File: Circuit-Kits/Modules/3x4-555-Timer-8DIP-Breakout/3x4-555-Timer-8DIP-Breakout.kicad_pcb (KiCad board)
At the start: 2 copper layers, 23.6 x 31.6 mm, 1 part, among them U1 555TIMER

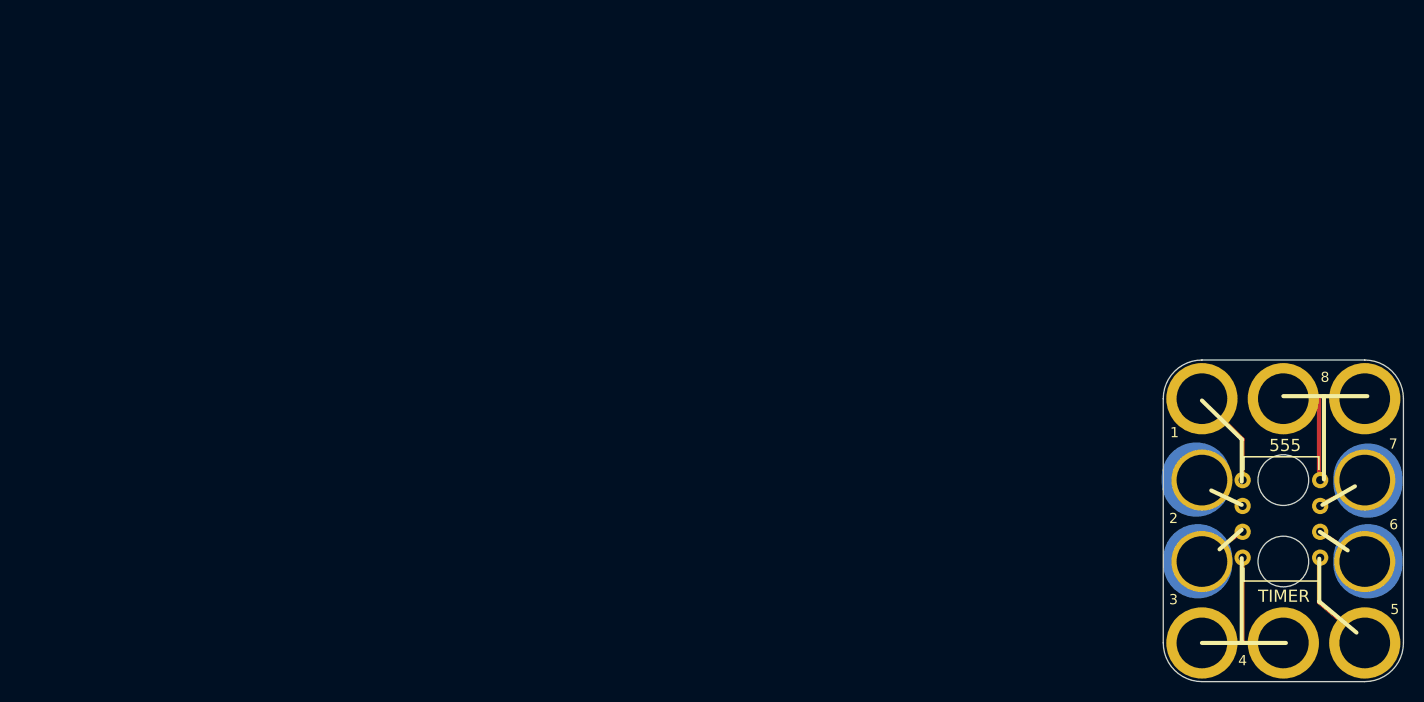
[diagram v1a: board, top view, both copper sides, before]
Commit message: Public release
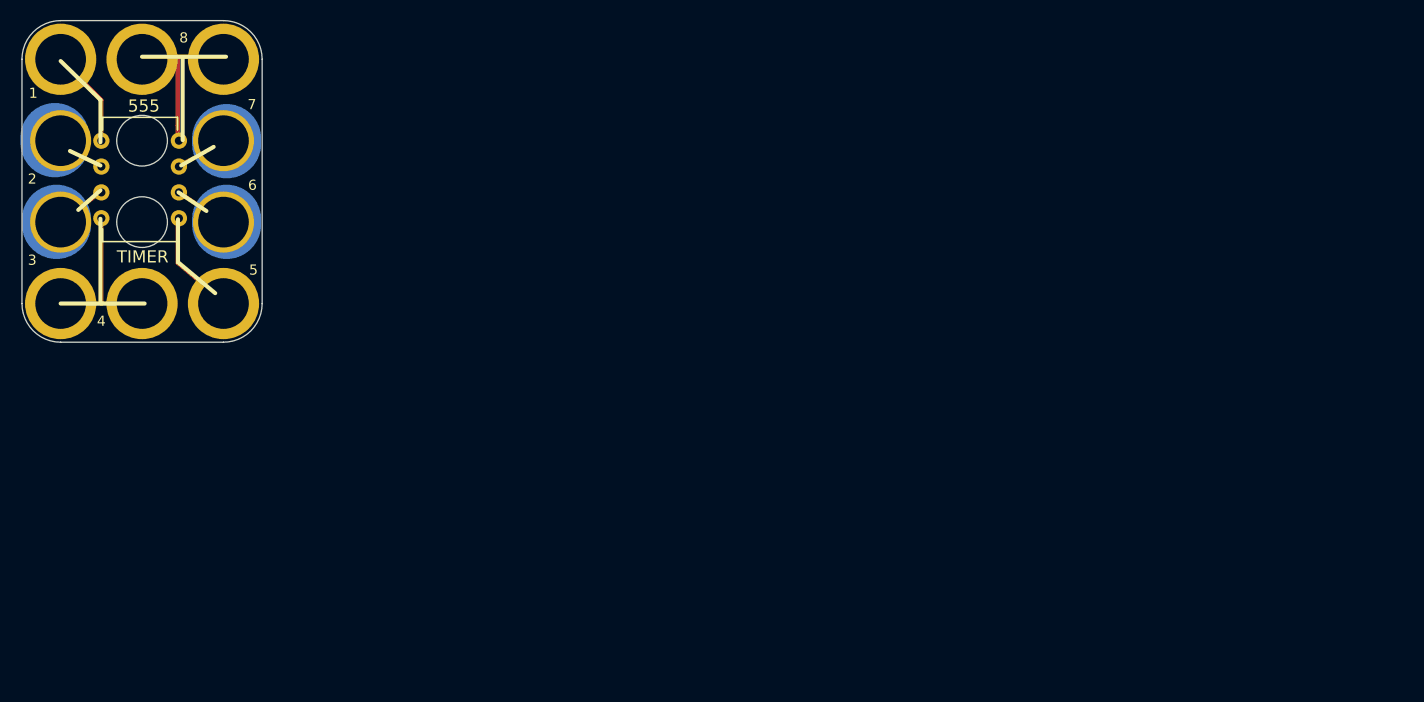
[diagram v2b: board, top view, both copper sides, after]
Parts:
- moved U1 117.0 mm to (22.8, 74.2)
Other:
- board text added: "FABRICATION NOTES 1. THIS IS A 2 LAYER BOARD. 2. EXTERNAL LAYERS SHALL HAVE 1 OZ COPPER. 3. MATERIAL: FR4 AND 0.062 INCH +/- 10% THICK. 4. BOARDS SHALL BE ROHS COMPLIANT. 5. MANUFACTURE IN ACCORDANCE WITH IPC-6012 CLASS 2 6. MASK: BOTH SIDES OF THE BOARD SHALL HAVE SOLDER MASK (GREEN) OVER BARE COPPER. 7. SILK: BOTH SIDES OF THE BOARD SHALL HAVE WHITE SILK. DO NOT PLACE SILK OVER BARE COPPER. 8. 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"
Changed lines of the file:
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@@
     (links 10)
     (no_connects 10)
-    (area 0 0 0 0)
+    (area 104.572999 74.854999 178.510001 123.265001)
     (thickness 1.6)
-    (drawings 18)
+    (drawings 2)
     (tracks 0)
     (zones 0)
@@
   )
   (module Crazy_Circuits:DIP8-3x4 (layer F.Cu)
-    (at 134.92172 107.50296)
+    (at 22.78072 74.15276)
     (descr "8-lead dip package, row spacing 7.62 mm (300 mils)")
     (tags "dil dip 2.54 300")
@@
     )
   )
-  (gr_text TIMER (at 142.98168 102.91064) (layer F.SilkS)
+  (gr_text "FABRICATION NOTES\n\n1. THIS IS A 2 LAYER BOARD. \n2. EXTERNAL LAYERS SHALL HAVE 1 OZ COPPER.\n3. MATERIAL: FR4 AND 0.062 INCH +/- 10% THICK.\n4. BOARDS SHALL BE ROHS COMPLIANT. \n5. MANUFACTURE IN ACCORDANCE WITH IPC-6012 CLASS 2\n6. MASK: BOTH SIDES OF THE BOARD SHALL HAVE \n   SOLDER MASK (GREEN) OVER BARE COPPER. \n7. SILK: BOTH SIDES OF THE BOARD SHALL HAVE WHITE SILK. \n   DO NOT PLACE SILK OVER BARE COPPER.\n8. FINISH: ENIG.\n9. MINIMUM TRACE WIDTH - 0.006 INCH.\n   MINIMUM SPACE - 0.006 INCH.\n   MINIMUM HOLE DIA - 0.013 INCH. \n10. MAX HOLE PLACEMENT TOLERANCE OF +/- 0.003 INCH.\n11. MAX HOLE DIAMETER TOLERANCE OF +/- 0.003 INCH AFTER PLATING." (at 0.127 124.4854) (layer Dwgs.User)
+    (effects (font (size 2.54 2.54) (thickness 0.254)) (justify left))
+  )
+  (gr_text TIMER (at 30.84068 69.56044) (layer F.SilkS)
     (effects (font (size 1.2 1.2) (thickness 0.2)))
   )
-  (gr_circle (center 117.348 76.962) (end 118.618 76.962) (layer Dwgs.User) (width 0.15))
-  (gr_line (start 114.427 78.994) (end 114.427 74.93) (angle 90) (layer Dwgs.User) (width 0.15))
-  (gr_line (start 120.269 78.994) (end 114.427 78.994) (angle 90) (layer Dwgs.User) (width 0.15))
-  (gr_line (start 120.269 74.93) (end 120.269 78.994) (angle 90) (layer Dwgs.User) (width 0.15))
-  (gr_line (start 114.427 74.93) (end 120.269 74.93) (angle 90) (layer Dwgs.User) (width 0.15))
-  (gr_line (start 120.523 93.98) (end 104.648 93.98) (angle 90) (layer Dwgs.User) (width 0.15))
-  (gr_line (start 173.355 102.235) (end 173.355 94.615) (angle 90) (layer Dwgs.User) (width 0.15))
-  (gr_line (start 178.435 102.235) (end 173.355 102.235) (angle 90) (layer Dwgs.User) (width 0.15))
-  (gr_line (start 178.435 94.615) (end 178.435 102.235) (angle 90) (layer Dwgs.User) (width 0.15))
-  (gr_line (start 173.355 94.615) (end 178.435 94.615) (angle 90) (layer Dwgs.User) (width 0.15))
-  (gr_line (start 109.093 123.19) (end 109.093 114.3) (angle 90) (layer Dwgs.User) (width 0.15))
-  (gr_line (start 122.428 123.19) (end 109.093 123.19) (angle 90) (layer Dwgs.User) (width 0.15))
-  (gr_line (start 122.428 114.3) (end 122.428 123.19) (angle 90) (layer Dwgs.User) (width 0.15))
-  (gr_line (start 109.093 114.3) (end 122.428 114.3) (angle 90) (layer Dwgs.User) (width 0.15))
-  (gr_line (start 104.648 93.98) (end 104.648 82.55) (angle 90) (layer Dwgs.User) (width 0.15))
-  (gr_line (start 120.523 82.55) (end 120.523 93.98) (angle 90) (layer Dwgs.User) (width 0.15))
-  (gr_line (start 104.648 82.55) (end 120.523 82.55) (angle 90) (layer Dwgs.User) (width 0.15))
 )
